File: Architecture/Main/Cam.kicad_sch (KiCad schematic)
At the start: 30 parts, among them J2 Screw_Terminal_01x02, J3 Conn_01x08, J7 Screw_Terminal_01x02, J8 Conn_02x08_Counter_Clockwise, Q3 NPN

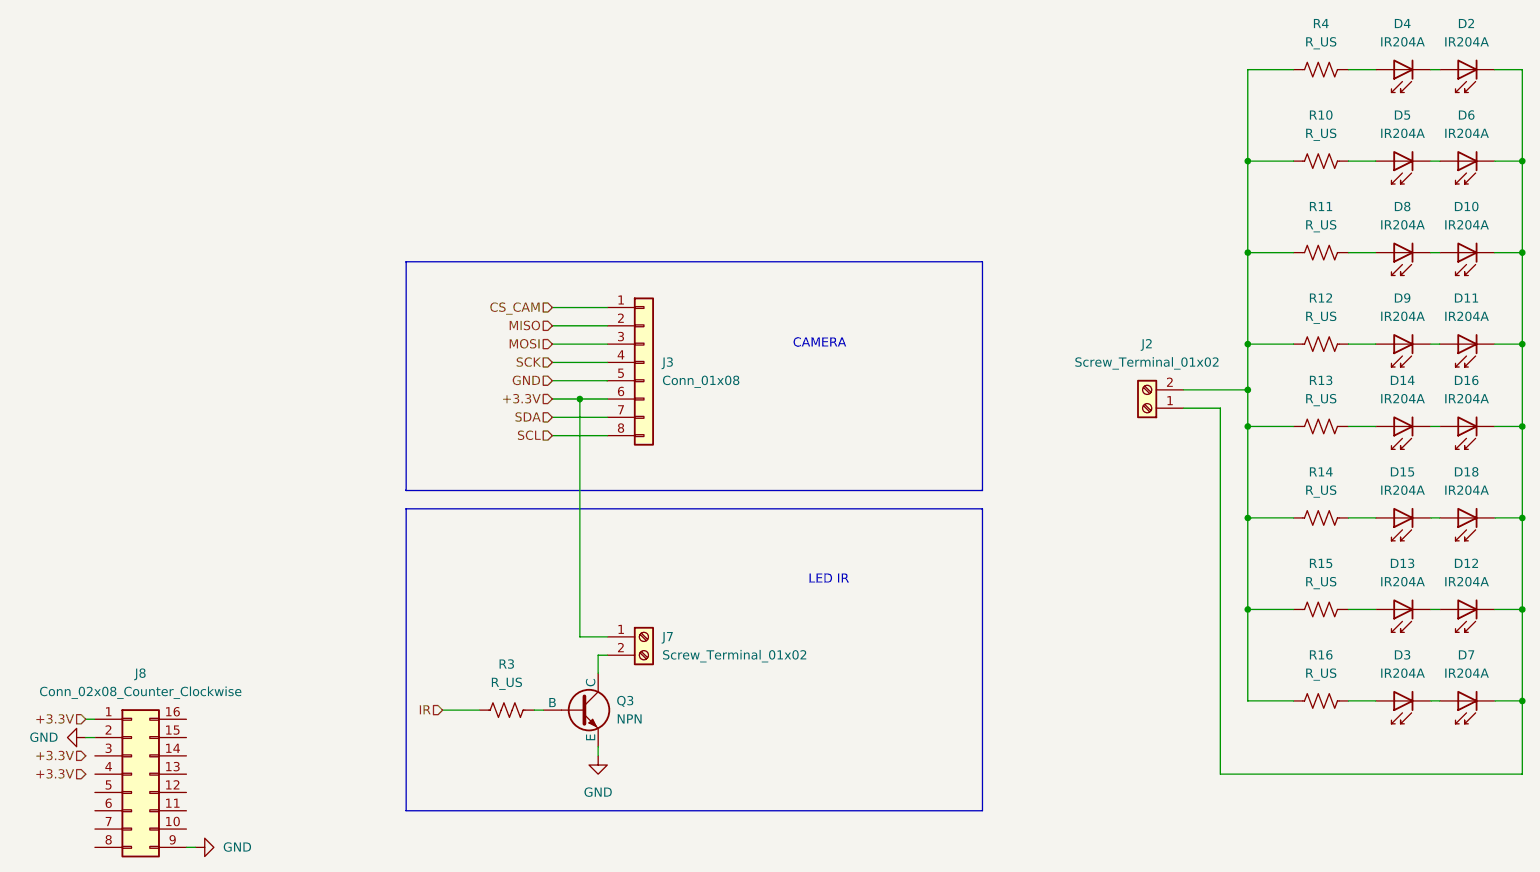
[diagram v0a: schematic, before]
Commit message: Update Schematic
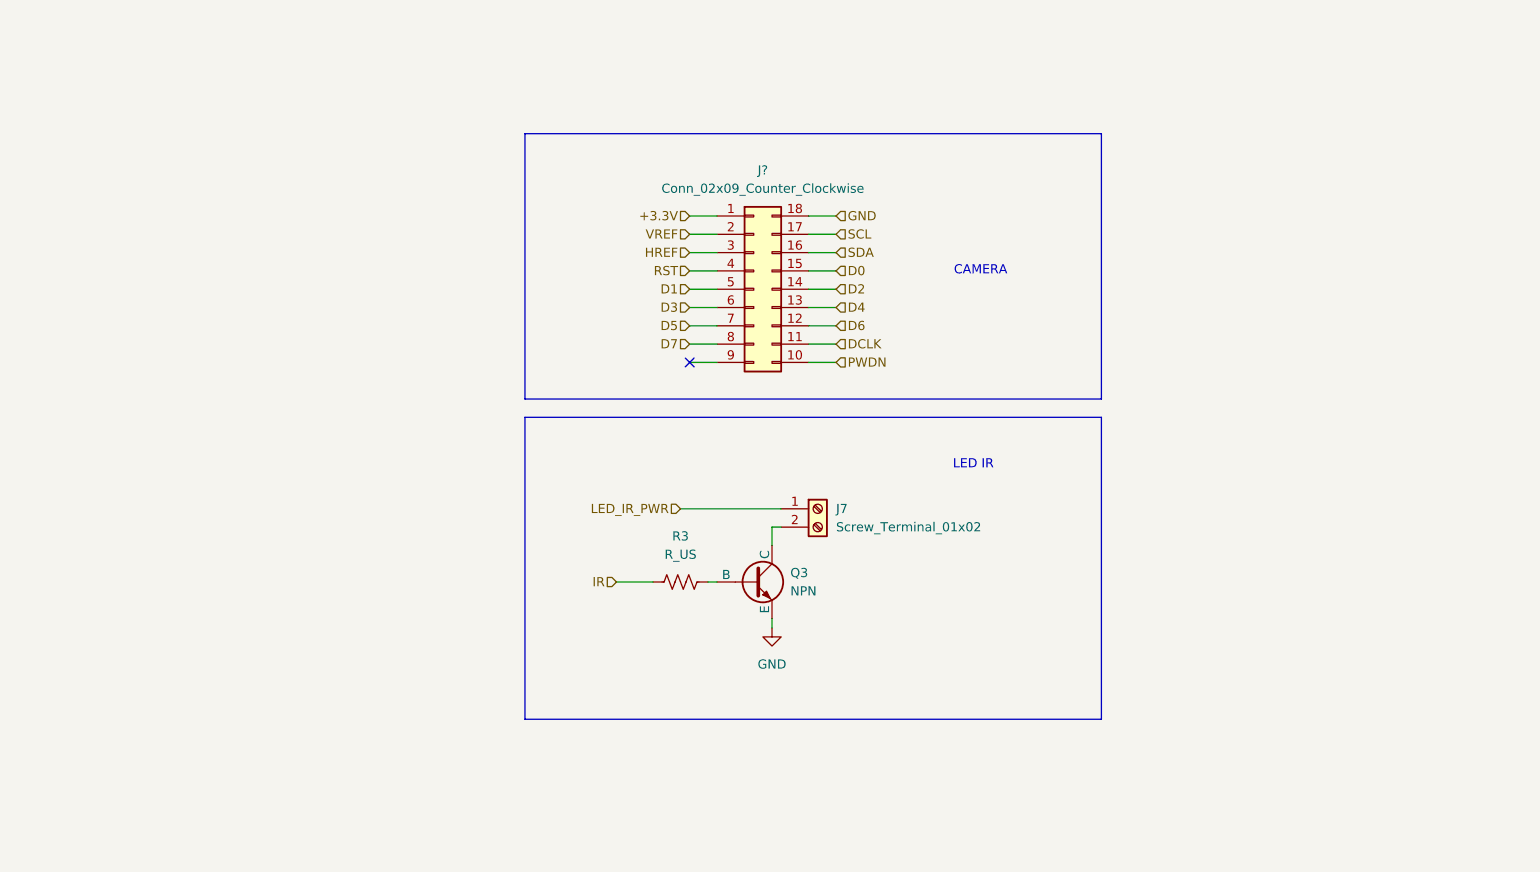
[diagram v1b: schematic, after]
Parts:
- removed D10, D11, D12, D13, D14, D15, D16, D18, D2, D3, D4, D5, D6, D7, D8, D9: IR204A, LED_THT:LED_D3.0mm_IRBlack, symbol LED:IR204A
- removed J2: Screw_Terminal_01x02, symbol Connector:Screw_Terminal_01x02
- removed J3: Conn_01x08, symbol Connector_Generic:Conn_01x08
- removed J8: Conn_02x08_Counter_Clockwise, symbol Connector_Generic:Conn_02x08_Counter_Clockwise
- removed R10, R11, R12, R13, R14, R15, R16: R_US, Resistor_SMD:R_0805_2012Metric_Pad1.20x1.40mm_HandSolder, symbol Device:R_US
- removed R4: R_US, symbol Device:R_US
- added J?: Conn_02x09_Counter_Clockwise, symbol Connector_Generic:Conn_02x09_Counter_Clockwise
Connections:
- net +3.3V: now also J?.1 (Pin_1); no longer J7.1 (Pin_1)
- net GND: now also J?.18 (Pin_18)
- net SCL: now also J?.17 (Pin_17)
- net SDA: now also J?.16 (Pin_16)
- new net D0: J?.15 (Pin_15)
- new net D1: J?.5 (Pin_5)
- new net D2: J?.14 (Pin_14)
- new net D3: J?.6 (Pin_6)
- new net D4: J?.13 (Pin_13)
- new net D5: J?.7 (Pin_7)
- new net D6: J?.12 (Pin_12)
- new net D7: J?.8 (Pin_8)
- new net DCLK: J?.11 (Pin_11)
- new net HREF: J?.3 (Pin_3)
- new net LED_IR_PWR: J7.1 (Pin_1)
- new net PWDN: J?.10 (Pin_10)
- new net RST: J?.4 (Pin_4)
- new net VREF: J?.2 (Pin_2)
- no-connect marks 0 -> 1
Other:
- moved on the sheet: J7, Q3, R3

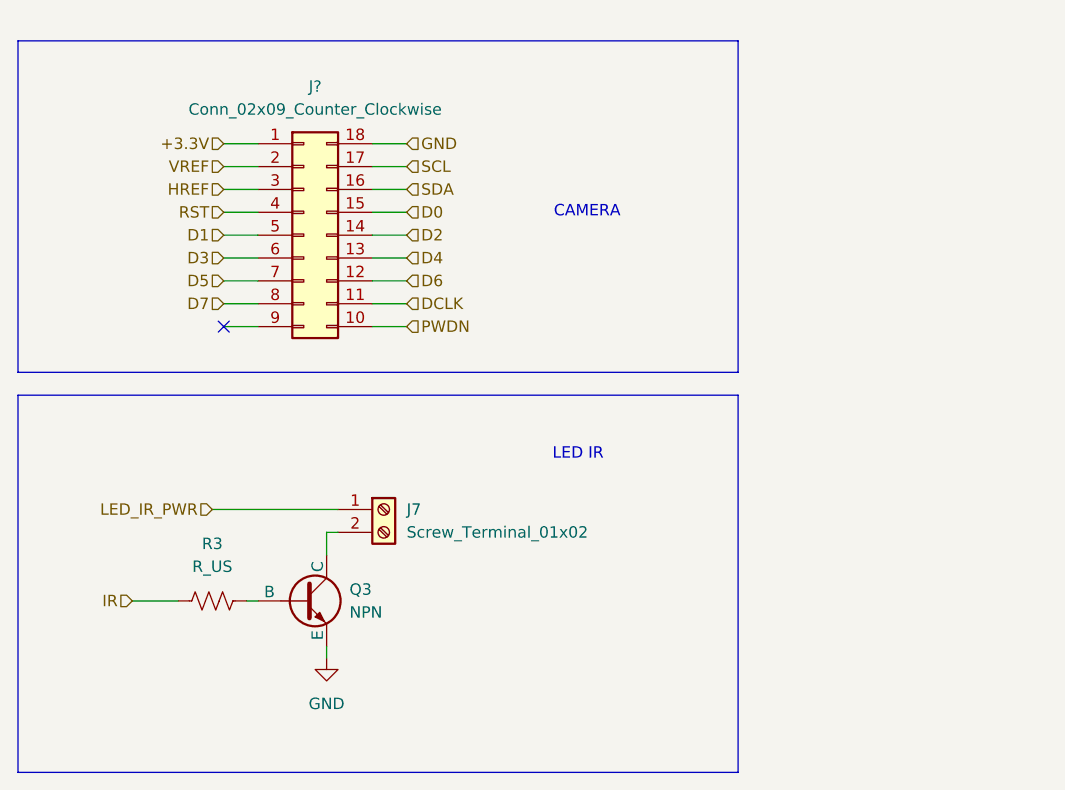
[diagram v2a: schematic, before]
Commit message: update
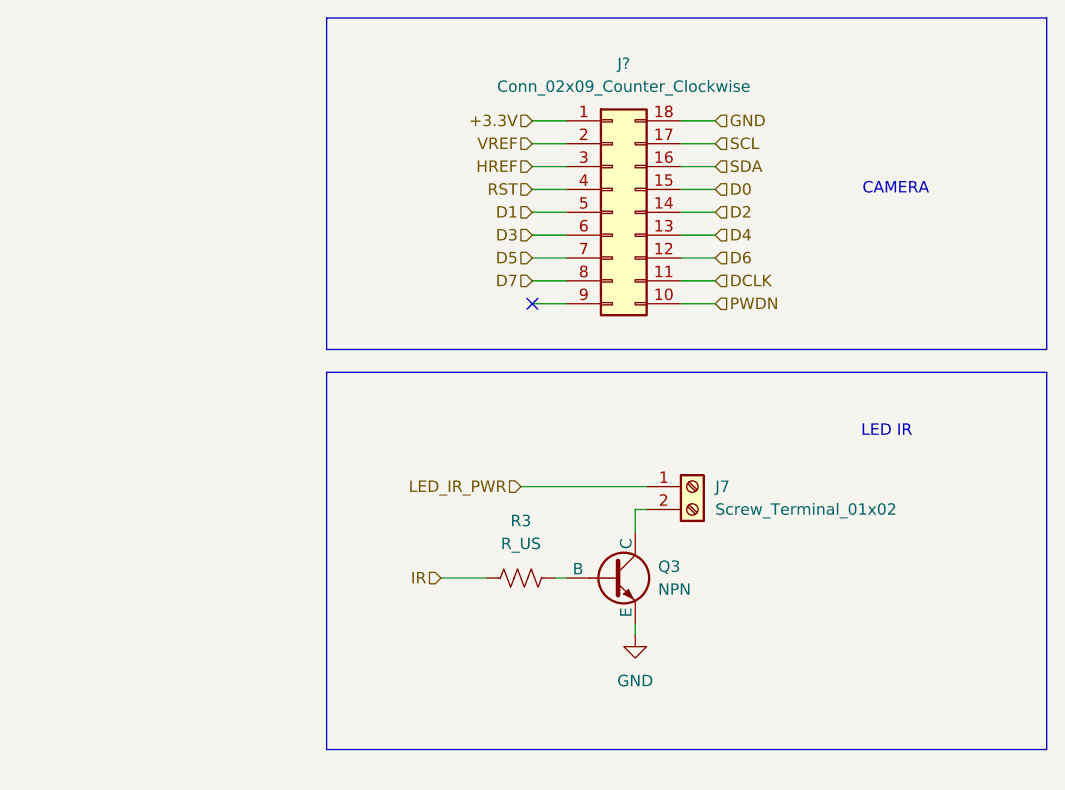
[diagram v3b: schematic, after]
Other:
- moved on the sheet: J7, J?, Q3, R3

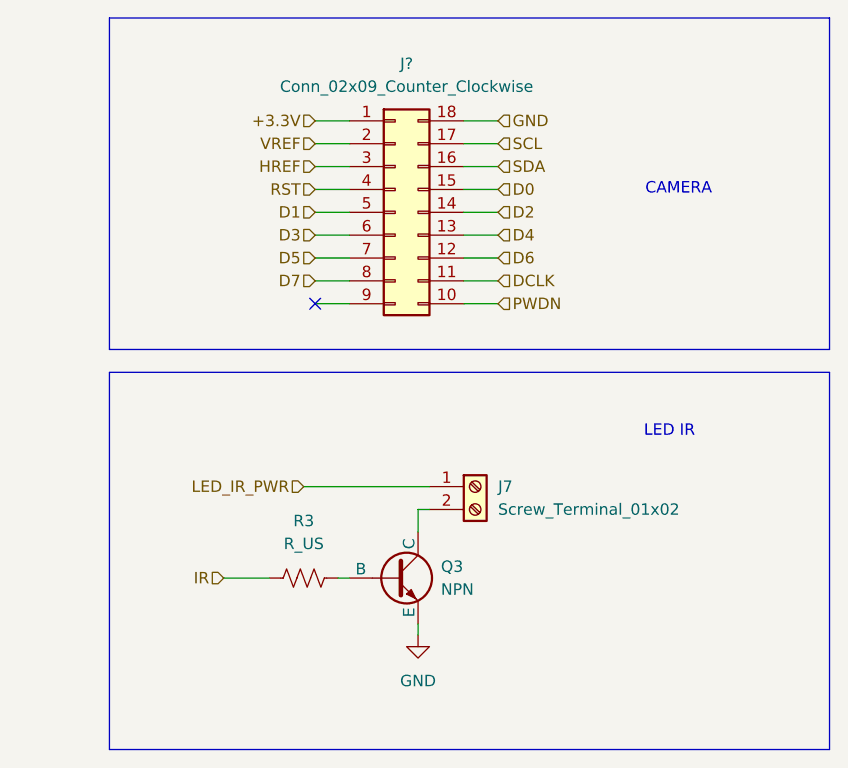
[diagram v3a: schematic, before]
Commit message: Update_07_01_2026
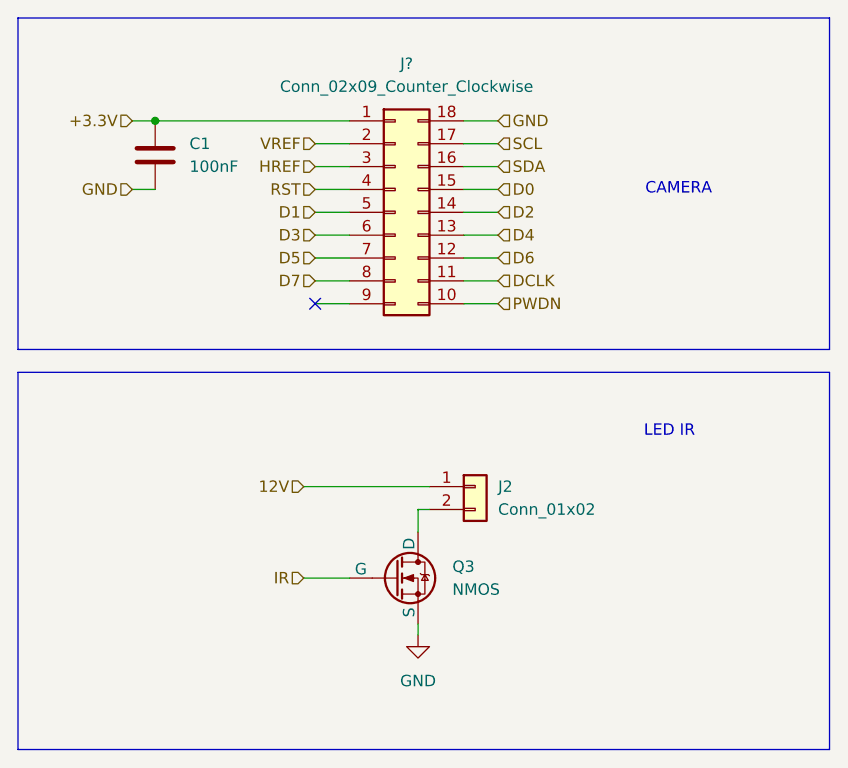
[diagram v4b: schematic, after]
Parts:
- removed J7: Screw_Terminal_01x02, symbol Connector:Screw_Terminal_01x02
- removed Q3: NPN, symbol Simulation_SPICE:NPN
- removed R3: R_US, symbol Device:R_US
- added C1: 100nF, symbol Device:C
- added J2: Conn_01x02, symbol Connector_Generic:Conn_01x02
- added Q3: NMOS, symbol Simulation_SPICE:NMOS
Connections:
- net +3.3V: now also C1.1
- net GND: now also C1.2, Q3.3 (S)
- net IR: now also Q3.2 (G)
- new net: J2.2 (Pin_2), Q3.1 (D)
- new net 12V: J2.1 (Pin_1)
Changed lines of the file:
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@@
 	(paper "A4")
 	(rectangle
-		(start 149.86 92.71)
+		(start 139.7 92.71)
 		(end 229.87 134.62)
 		(stroke
@@
 	)
 	(rectangle
-		(start 149.86 53.34)
+		(start 139.7 53.34)
 		(end 229.87 90.17)
 		(stroke
@@
 		)
 	)
+	(junction
+		(at 154.94 64.77)
+		(diameter 0)
+		(color 0 0 0 0)
+	)
 	(no_connect
 		(at 172.72 85.09)
@@
 	(wire
 		(pts
-			(xy 162.56 115.57) (xy 167.64 115.57)
+			(xy 171.45 115.57) (xy 176.53 115.57)
 		)
 		(stroke
@@
 	(wire
 		(pts
-			(xy 175.26 115.57) (xy 176.53 115.57)
+			(xy 189.23 82.55) (xy 193.04 82.55)
 		)
 		(stroke
@@
 	(wire
 		(pts
-			(xy 189.23 82.55) (xy 193.04 82.55)
+			(xy 154.94 64.77) (xy 176.53 64.77)
 		)
 		(stroke
@@
 	(wire
 		(pts
-			(xy 172.72 64.77) (xy 176.53 64.77)
+			(xy 152.4 64.77) (xy 154.94 64.77)
 		)
 		(stroke
@@
 	(wire
 		(pts
+			(xy 152.4 72.39) (xy 154.94 72.39)
+		)
+		(stroke
+			(width 0)
+			(type default)
+		)
+	)
+	(wire
+		(pts
 			(xy 172.72 82.55) (xy 176.53 82.55)
 		)
@@
 		)
 	)
+	(hierarchical_label "GND"
+		(shape input)
+		(at 152.4 72.39 180)
+		(effects
+			(font
+				(size 1.27 1.27)
+			)
+			(justify right)
+		)
+	)
 	(hierarchical_label "IR"
 		(shape input)
-		(at 162.56 115.57 180)
+		(at 171.45 115.57 180)
 		(effects
 			(font
@@
 	(hierarchical_label "+3.3V"
 		(shape input)
-		(at 172.72 64.77 180)
+		(at 152.4 64.77 180)
 		(effects
 			(font
@@
 		)
 	)
-	(hierarchical_label "LED_IR_PWR"
+	(hierarchical_label "D7"
 		(shape input)
-		(at 171.45 105.41 180)
+		(at 172.72 82.55 180)
 		(effects
 			(font
@@
 		)
 	)
-	(hierarchical_label "D7"
+	(hierarchical_label "12V"
 		(shape input)
-		(at 172.72 82.55 180)
+		(at 171.45 105.41 180)
 		(effects
 			(font
@@
 	)
 	(symbol
-		(lib_id "Connector:Screw_Terminal_01x02")
+		(lib_id "Connector_Generic:Conn_01x02")
 		(at 190.5 105.41 0)
 		(unit 1)
@@
 		(dnp no)
 		(fields_autoplaced yes)
-		(property "Reference" "J7"
+		(property "Reference" "J2"
 			(at 193.04 105.4099 0)
 			(effects
@@
 			)
 		)
-		(property "Value" "Screw_Terminal_01x02"
+		(property "Value" "Conn_01x02"
 			(at 193.04 107.9499 0)
 			(effects
@@
 			)
 		)
-		(property "Description" "Generic screw terminal, single row, 01x02, script generated (kicad-library-utils/schlib/autogen/connector/)"
+		(property "Description" "Generic connector, single row, 01x02, script generated (kicad-library-utils/schlib/autogen/connector/)"
 			(at 190.5 105.41 0)
 			(effects
@@
 			)
 		)
-		(pin "2"
-		)
 		(pin "1"
 		)
+		(pin "2"
+		)
 		(instances
 			(project ""
 				(path "/77f264da-4c84-4b0c-9d20-4392731765e6/90e676b5-e192-40ef-8f2d-7a9315f03418"
-					(reference "J7")
-					(unit 1)
-				)
-			)
-			(project "Cam"
-				(path "/7fd1e59d-d896-4263-8d21-df7365fed559"
-					(reference "J?")
+					(reference "J2")
 					(unit 1)
 				)
@@
 	)
 	(symbol
-		(lib_id "Device:R_US")
-		(at 171.45 115.57 90)
+		(lib_id "Simulation_SPICE:NMOS")
+		(at 181.61 115.57 0)
 		(unit 1)
 		(exclude_from_sim no)
@@
 		(dnp no)
 		(fields_autoplaced yes)
-		(property "Reference" "R3"
-			(at 171.45 109.22 90)
+		(property "Reference" "Q3"
+			(at 187.96 114.2999 0)
 			(effects
 				(font
 					(size 1.27 1.27)
 				)
+				(justify left)
 			)
 		)
-		(property "Value" "R_US"
-			(at 171.45 111.76 90)
+		(property "Value" "NMOS"
+			(at 187.96 116.8399 0)
 			(effects
 				(font
 					(size 1.27 1.27)
 				)
+				(justify left)
 			)
 		)
 		(property "Footprint" ""
-			(at 171.704 114.554 90)
+			(at 186.69 113.03 0)
 			(effects
 				(font
@@
 			)
 		)
-		(property "Datasheet" "~"
-			(at 171.45 115.57 0)
+		(property "Datasheet" "https://ngspice.sourceforge.io/docs/ngspice-html-manual/manual.xhtml#cha_MOSFETs"
+			(at 181.61 128.27 0)
+			(effects
+				(font
+					(size 1.27 1.27)
+				)
+				(hide yes)
+			)
+		)
+		(property "Description" "N-MOSFET transistor, drain/source/gate"
+			(at 181.61 115.57 0)
 			(effects
 				(font
@@
 			)
 		)
-		(property "Description" "Resistor, US symbol"
-			(at 171.45 115.57 0)
+		(property "Sim.Device" "NMOS"
+			(at 181.61 132.715 0)
 			(effects
 				(font
@@
 			)
 		)
-		(pin "1"
+		(property "Sim.Type" "VDMOS"
+			(at 181.61 134.62 0)
+			(effects
+				(font
+					(size 1.27 1.27)
+				)
+				(hide yes)
+			)
+		)
+		(property "Sim.Pins" "1=D 2=G 3=S"
+			(at 181.61 130.81 0)
+			(effects
+				(font
+					(size 1.27 1.27)
+				)
+				(hide yes)
+			)
+		)
+		(pin "3"
 		)
 		(pin "2"
 		)
+		(pin "1"
+		)
 		(instances
 			(project ""
 				(path "/77f264da-4c84-4b0c-9d20-4392731765e6/90e676b5-e192-40ef-8f2d-7a9315f03418"
-					(reference "R3")
-					(unit 1)
-				)
-			)
-			(project "Cam"
-				(path "/7fd1e59d-d896-4263-8d21-df7365fed559"
-					(reference "R?")
+					(reference "Q3")
 					(unit 1)
 				)
@@
 	)
 	(symbol
-		(lib_id "Simulation_SPICE:NPN")
-		(at 181.61 115.57 0)
+		(lib_id "Device:C")
+		(at 154.94 68.58 0)
 		(unit 1)
 		(exclude_from_sim no)
@@
 		(dnp no)
 		(fields_autoplaced yes)
-		(property "Reference" "Q3"
-			(at 186.69 114.2999 0)
+		(property "Reference" "C1"
+			(at 158.75 67.3099 0)
 			(effects
 				(font
@@
 			)
 		)
-		(property "Value" "NPN"
-			(at 186.69 116.8399 0)
+		(property "Value" "100nF"
+			(at 158.75 69.8499 0)
 			(effects
 				(font
@@
 		)
 		(property "Footprint" ""
-			(at 245.11 115.57 0)
-			(effects
-				(font
-					(size 1.27 1.27)
-				)
-				(hide yes)
-			)
-		)
-		(property "Datasheet" "https://ngspice.sourceforge.io/docs/ngspice-html-manual/manual.xhtml#cha_BJTs"
-			(at 245.11 115.57 0)
-			(effects
-				(font
-					(size 1.27 1.27)
-				)
-				(hide yes)
-			)
-		)
-		(property "Description" "Bipolar transistor symbol for simulation only, substrate tied to the emitter"
-			(at 181.61 115.57 0)
-			(effects
-				(font
-					(size 1.27 1.27)
-				)
-				(hide yes)
-			)
-		)
-		(property "Sim.Device" "NPN"
-			(at 181.61 115.57 0)
+			(at 155.9052 72.39 0)
 			(effects
 				(font
@@
 			)
 		)
-		(property "Sim.Type" "GUMMELPOON"
-			(at 181.61 115.57 0)
+		(property "Datasheet" "~"
+			(at 154.94 68.58 0)
 			(effects
 				(font
@@
 			)
 		)
-		(property "Sim.Pins" "1=C 2=B 3=E"
-			(at 181.61 115.57 0)
+		(property "Description" "Unpolarized capacitor"
+			(at 154.94 68.58 0)
 			(effects
 				(font
@@
 			)
 		)
-		(pin "3"
+		(pin "1"
 		)
 		(pin "2"
 		)
-		(pin "1"
-		)
 		(instances
 			(project ""
 				(path "/77f264da-4c84-4b0c-9d20-4392731765e6/90e676b5-e192-40ef-8f2d-7a9315f03418"
-					(reference "Q3")
-					(unit 1)
-				)
-			)
-			(project "Cam"
-				(path "/7fd1e59d-d896-4263-8d21-df7365fed559"
-					(reference "Q?")
+					(reference "C1")
 					(unit 1)
 				)
